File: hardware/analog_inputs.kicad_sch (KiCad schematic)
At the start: 0 parts

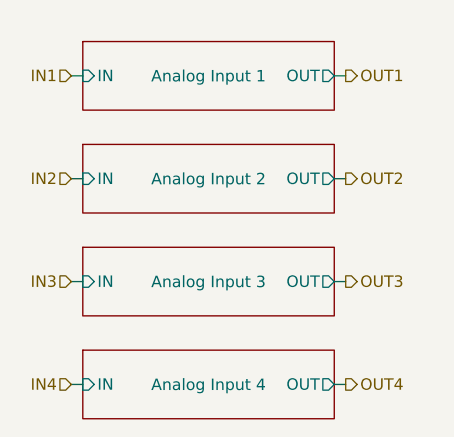
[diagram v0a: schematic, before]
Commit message: Add the Cube project
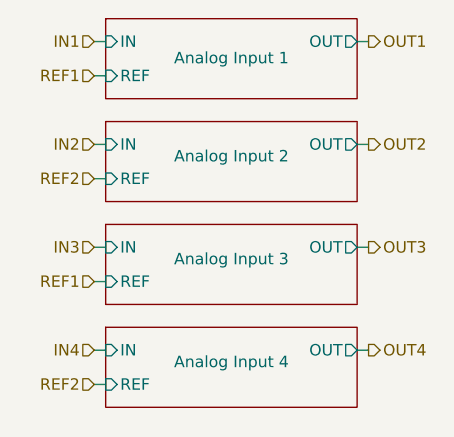
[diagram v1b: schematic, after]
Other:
- sheet Analog Input 1 ports: added REF; removed none
- sheet Analog Input 2 ports: added REF; removed none
- sheet Analog Input 3 ports: added REF; removed none
- sheet Analog Input 4 ports: added REF; removed none
- title: (none) -> Analog Inputs
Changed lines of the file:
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@@
   (paper "A4")
   (title_block
-    (date "2023-06-06")
+    (title "Analog Inputs")
+    (date "2023-07-01")
     (rev "${REVISION}")
     (company "Author: I. Kajdan")
     (comment 1 "Reviewer:")
   )
-  (wire (pts (xy 133.35 107.95) (xy 134.62 107.95))
+  (wire (pts (xy 135.89 104.14) (xy 137.16 104.14))
     (stroke (width 0) (type default))
   )
-  (wire (pts (xy 162.56 96.52) (xy 163.83 96.52))
+  (wire (pts (xy 165.1 92.71) (xy 166.37 92.71))
     (stroke (width 0) (type default))
   )
-  (wire (pts (xy 133.35 85.09) (xy 134.62 85.09))
+  (wire (pts (xy 135.89 107.95) (xy 137.16 107.95))
     (stroke (width 0) (type default))
   )
-  (wire (pts (xy 162.56 119.38) (xy 163.83 119.38))
+  (wire (pts (xy 135.89 81.28) (xy 137.16 81.28))
     (stroke (width 0) (type default))
   )
-  (wire (pts (xy 133.35 119.38) (xy 134.62 119.38))
+  (wire (pts (xy 165.1 115.57) (xy 166.37 115.57))
     (stroke (width 0) (type default))
   )
-  (wire (pts (xy 162.56 85.09) (xy 163.83 85.09))
+  (wire (pts (xy 135.89 115.57) (xy 137.16 115.57))
     (stroke (width 0) (type default))
   )
-  (wire (pts (xy 162.56 107.95) (xy 163.83 107.95))
+  (wire (pts (xy 135.89 96.52) (xy 137.16 96.52))
     (stroke (width 0) (type default))
   )
-  (wire (pts (xy 133.35 96.52) (xy 134.62 96.52))
+  (wire (pts (xy 135.89 119.38) (xy 137.16 119.38))
     (stroke (width 0) (type default))
   )
-  (hierarchical_label "IN4" (shape input) (at 133.35 119.38 180) (fields_autoplaced)
+  (wire (pts (xy 165.1 81.28) (xy 166.37 81.28))
+    (stroke (width 0) (type default))
+  )
+  (wire (pts (xy 135.89 85.09) (xy 137.16 85.09))
+    (stroke (width 0) (type default))
+  )
+  (wire (pts (xy 165.1 104.14) (xy 166.37 104.14))
+    (stroke (width 0) (type default))
+  )
+  (wire (pts (xy 135.89 92.71) (xy 137.16 92.71))
+    (stroke (width 0) (type default))
+  )
+  (hierarchical_label "REF1" (shape input) (at 135.89 107.95 180) (fields_autoplaced)
     (effects (font (size 1.27 1.27)) (justify right))
   )
-  (hierarchical_label "OUT2" (shape output) (at 163.83 96.52 0) (fields_autoplaced)
+  (hierarchical_label "IN4" (shape input) (at 135.89 115.57 180) (fields_autoplaced)
+    (effects (font (size 1.27 1.27)) (justify right))
+  )
+  (hierarchical_label "OUT2" (shape output) (at 166.37 92.71 0) (fields_autoplaced)
     (effects (font (size 1.27 1.27)) (justify left))
   )
-  (hierarchical_label "OUT4" (shape output) (at 163.83 119.38 0) (fields_autoplaced)
+  (hierarchical_label "REF2" (shape input) (at 135.89 96.52 180) (fields_autoplaced)
+    (effects (font (size 1.27 1.27)) (justify right))
+  )
+  (hierarchical_label "OUT4" (shape output) (at 166.37 115.57 0) (fields_autoplaced)
     (effects (font (size 1.27 1.27)) (justify left))
   )
-  (hierarchical_label "IN3" (shape input) (at 133.35 107.95 180) (fields_autoplaced)
+  (hierarchical_label "REF2" (shape input) (at 135.89 119.38 180) (fields_autoplaced)
     (effects (font (size 1.27 1.27)) (justify right))
   )
-  (hierarchical_label "OUT3" (shape output) (at 163.83 107.95 0) (fields_autoplaced)
+  (hierarchical_label "REF1" (shape input) (at 135.89 85.09 180) (fields_autoplaced)
+    (effects (font (size 1.27 1.27)) (justify right))
+  )
+  (hierarchical_label "IN3" (shape input) (at 135.89 104.14 180) (fields_autoplaced)
+    (effects (font (size 1.27 1.27)) (justify right))
+  )
+  (hierarchical_label "OUT3" (shape output) (at 166.37 104.14 0) (fields_autoplaced)
     (effects (font (size 1.27 1.27)) (justify left))
   )
-  (hierarchical_label "IN1" (shape input) (at 133.35 85.09 180) (fields_autoplaced)
+  (hierarchical_label "IN1" (shape input) (at 135.89 81.28 180) (fields_autoplaced)
     (effects (font (size 1.27 1.27)) (justify right))
   )
-  (hierarchical_label "OUT1" (shape output) (at 163.83 85.09 0) (fields_autoplaced)
+  (hierarchical_label "OUT1" (shape output) (at 166.37 81.28 0) (fields_autoplaced)
     (effects (font (size 1.27 1.27)) (justify left))
   )
-  (hierarchical_label "IN2" (shape input) (at 133.35 96.52 180) (fields_autoplaced)
+  (hierarchical_label "IN2" (shape input) (at 135.89 92.71 180) (fields_autoplaced)
     (effects (font (size 1.27 1.27)) (justify right))
   )
-  (sheet (at 134.62 81.28) (size 27.94 7.62)
+  (sheet (at 137.16 78.74) (size 27.94 8.89)
     (stroke (width 0.1524) (type solid))
     (fill (color 0 0 0 0.0000))
-    (property "Sheetname" "Analog Input 1" (at 148.59 84.3784 0)
-      (effects (font (size 1.27 1.27)) (justify top))
+    (property "Sheetname" "Analog Input 1" (at 151.13 83.1084 0)
+      (effects (font (size 1.27 1.27)))
     )
-    (property "Sheetfile" "analog_input.kicad_sch" (at 134.62 98.3746 0)
+    (property "Sheetfile" "analog_input.kicad_sch" (at 137.16 95.8346 0)
       (effects (font (size 1.27 1.27)) (justify left top) hide)
     )
-    (pin "IN" input (at 134.62 85.09 180)
+    (pin "IN" input (at 137.16 81.28 180)
       (effects (font (size 1.27 1.27)) (justify left))
     )
-    (pin "OUT" output (at 162.56 85.09 0)
+    (pin "OUT" output (at 165.1 81.28 0)
       (effects (font (size 1.27 1.27)) (justify right))
+    )
+    (pin "REF" input (at 137.16 85.09 180)
+      (effects (font (size 1.27 1.27)) (justify left))
     )
     (instances
@@
     )
   )
-  (sheet (at 134.62 104.14) (size 27.94 7.62)
+  (sheet (at 137.16 101.6) (size 27.94 8.89)
     (stroke (width 0.1524) (type solid))
     (fill (color 0 0 0 0.0000))
-    (property "Sheetname" "Analog Input 3" (at 148.59 107.2384 0)
+    (property "Sheetname" "Analog Input 3" (at 151.13 104.6984 0)
       (effects (font (size 1.27 1.27)) (justify top))
     )
-    (property "Sheetfile" "analog_input.kicad_sch" (at 134.62 121.2346 0)
+    (property "Sheetfile" "analog_input.kicad_sch" (at 137.16 118.6946 0)
       (effects (font (size 1.27 1.27)) (justify left top) hide)
     )
-    (pin "IN" input (at 134.62 107.95 180)
+    (pin "IN" input (at 137.16 104.14 180)
       (effects (font (size 1.27 1.27)) (justify left))
     )
-    (pin "OUT" output (at 162.56 107.95 0)
+    (pin "OUT" output (at 165.1 104.14 0)
       (effects (font (size 1.27 1.27)) (justify right))
+    )
+    (pin "REF" input (at 137.16 107.95 180)
+      (effects (font (size 1.27 1.27)) (justify left))
     )
     (instances
@@
     )
   )
-  (sheet (at 134.62 115.57) (size 27.94 7.62)
+  (sheet (at 137.16 113.03) (size 27.94 8.89)
     (stroke (width 0.1524) (type solid))
     (fill (color 0 0 0 0.0000))
-    (property "Sheetname" "Analog Input 4" (at 148.59 118.6684 0)
+    (property "Sheetname" "Analog Input 4" (at 151.13 116.1284 0)
       (effects (font (size 1.27 1.27)) (justify top))
     )
-    (property "Sheetfile" "analog_input.kicad_sch" (at 134.62 132.6646 0)
+    (property "Sheetfile" "analog_input.kicad_sch" (at 137.16 130.1246 0)
       (effects (font (size 1.27 1.27)) (justify left top) hide)
     )
-    (pin "IN" input (at 134.62 119.38 180)
+    (pin "IN" input (at 137.16 115.57 180)
       (effects (font (size 1.27 1.27)) (justify left))
     )
-    (pin "OUT" output (at 162.56 119.38 0)
+    (pin "OUT" output (at 165.1 115.57 0)
       (effects (font (size 1.27 1.27)) (justify right))
+    )
+    (pin "REF" input (at 137.16 119.38 180)
+      (effects (font (size 1.27 1.27)) (justify left))
     )
     (instances
@@
     )
   )
-  (sheet (at 134.62 92.71) (size 27.94 7.62)
+  (sheet (at 137.16 90.17) (size 27.94 8.89)
     (stroke (width 0.1524) (type solid))
     (fill (color 0 0 0 0.0000))
-    (property "Sheetname" "Analog Input 2" (at 148.59 95.8084 0)
+    (property "Sheetname" "Analog Input 2" (at 151.13 93.2684 0)
       (effects (font (size 1.27 1.27)) (justify top))
     )
-    (property "Sheetfile" "analog_input.kicad_sch" (at 134.62 109.8046 0)
+    (property "Sheetfile" "analog_input.kicad_sch" (at 137.16 107.2646 0)
       (effects (font (size 1.27 1.27)) (justify left top) hide)
     )
-    (pin "IN" input (at 134.62 96.52 180)
+    (pin "IN" input (at 137.16 92.71 180)
       (effects (font (size 1.27 1.27)) (justify left))
     )
-    (pin "OUT" output (at 162.56 96.52 0)
+    (pin "OUT" output (at 165.1 92.71 0)
       (effects (font (size 1.27 1.27)) (justify right))
     )
+    (pin "REF" input (at 137.16 96.52 180)
+      (effects (font (size 1.27 1.27)) (justify left))
+    )
     (instances
